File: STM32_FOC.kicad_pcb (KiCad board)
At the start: 2 copper layers, 26.5 x 26.5 mm, 46 parts, among them J1 Conn_01x07, J2 Conn_01x02, J3 Conn_01x03, J4 Conn_01x04, U1 STM32F103C8T6, U2 MP2359, U3 AS5600, U4 DRV8313, Y1 Crystal_GND3_Small

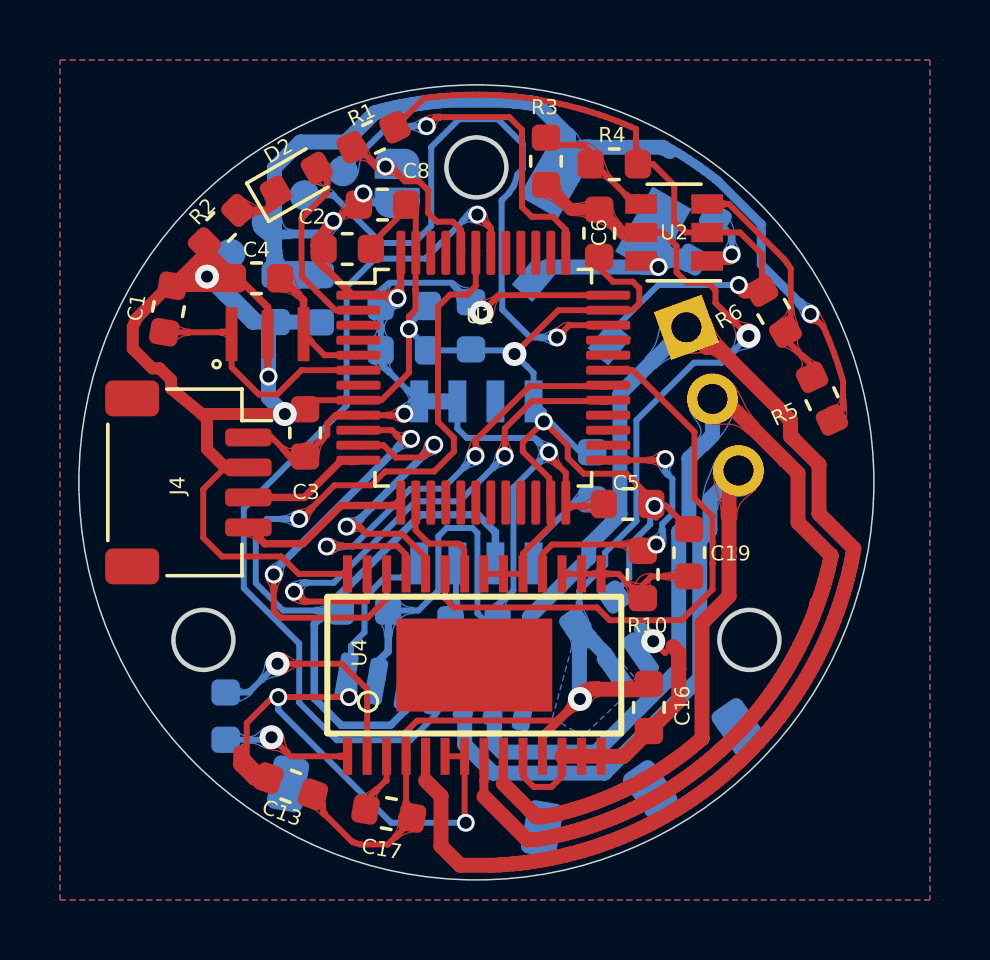
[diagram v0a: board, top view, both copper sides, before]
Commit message: first commit
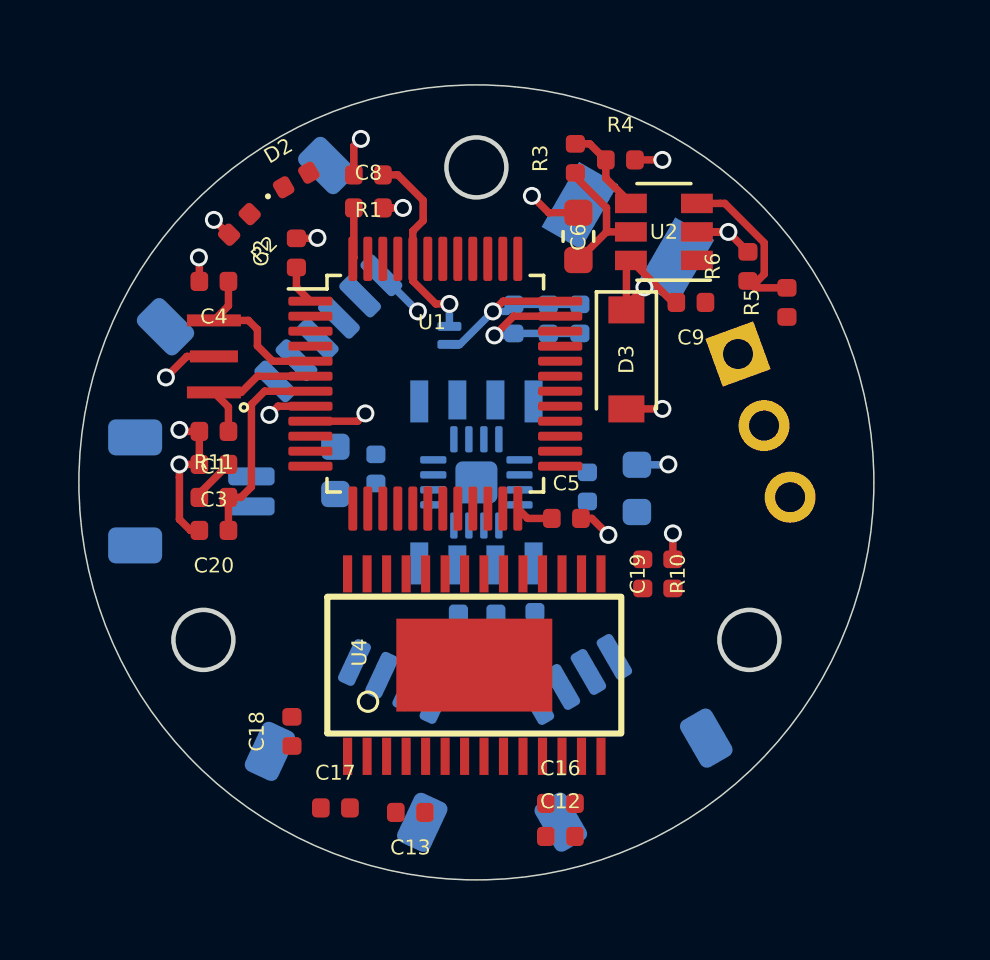
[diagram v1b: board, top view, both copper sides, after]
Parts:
- removed 3.3V, CLK, DIO, GND: TestPoint, TestPoint:TestPoint_Pad_D1.0mm
- added C20: 100nf, Capacitor_SMD:C_0402_1005Metric, F.Cu at (91.2, 101.6)
- added C21: 100nf, Capacitor_SMD:C_0402_1005Metric, B.Cu at (103.7, 100.2)
- added C22: 10uf, Capacitor_SMD:C_0603_1608Metric, B.Cu at (105.3, 100.2)
- added J5: Conn_01x06, Connector_JST:JST_SH_SM06B-SRSS-TB_1x06-1MP_P1.00mm_Horizontal, B.Cu at (93.7, 93.5)
- added R11: 10K, Resistor_SMD:R_0402_1005Metric, F.Cu at (91.2, 100.5)
- C1, C10, C11, C13, C16, C17, C2, C3, C4, C5, C7, C8: footprint Capacitor_SMD:C_0603_1608Metric -> Capacitor_SMD:C_0402_1005Metric
- C12, C18, C9: footprint Capacitor_SMD:C_0603_1608Metric -> Capacitor_SMD:C_0402_1005Metric; moved to F.Cu
- C14: value 0.1uf -> 100nf; footprint Capacitor_SMD:C_0603_1608Metric -> Capacitor_SMD:C_0402_1005Metric
- C19: value 100uf -> 0.47uf; footprint Capacitor_SMD:C_0603_1608Metric -> Capacitor_SMD:C_0402_1005Metric
- D2: footprint LED_SMD:LED_0603_1608Metric -> LED_SMD:LED_0402_1005Metric
- D3: moved to F.Cu
- J1: value Conn_01x07 -> Conn_01x04; footprint Connector_JST:JST_SH_SM07B-SRSS-TB_1x07-1MP_P1.00mm_Horizontal -> Connector_JST:JST_SH_SM04B-SRSS-TB_1x04-1MP_P1.00mm_Horizontal
- J4: moved to B.Cu
- JP1: footprint Jumper:SolderJumper-2_P1.3mm_Open_RoundedPad1.0x1.5mm -> Jumper:SoldJumper-2-P0.5mm_Open_RoundedPad
- R1, R10, R2, R3, R4, R5, R6, R7, R8, R9: footprint Resistor_SMD:R_0603_1608Metric -> Resistor_SMD:R_0402_1005Metric
- moved J2 17.3 mm to (90.5, 100.3), turned to 90 degrees
- moved J4 10.4 mm to (96.5, 108.5), turned to 155 degrees
- moved C11 10.2 mm to (103.5, 94.5)
- moved C10 7.65 mm to (102.4, 94.5)
- moved C12 7.62 mm to (102.8, 111.8), turned to 0 degrees
- moved J1 6.05 mm to (104.3, 108.3), turned to 210 degrees
- moved C15 5.94 mm to (95.3, 99.6), turned to 90 degrees
- moved R8 5.37 mm to (102.0, 104.8)
- moved JP1 5.34 mm to (99.0, 95.1)
- moved C1 4.35 mm to (91.2, 98.3), turned to 180 degrees
- moved C16 4.35 mm to (102.8, 110.7), turned to 0 degrees
- moved C13 4.08 mm to (97.8, 111.0), turned to 180 degrees
- moved C14 4.06 mm to (96.7, 99.5), turned to 90 degrees
- moved R5 3.42 mm to (110.3, 94.0), turned to 90 degrees
- moved C3 3.22 mm to (91.2, 99.4), turned to 180 degrees
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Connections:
- net Net-(U1-Pad32) renamed USB_DM
- net Net-(U1-Pad33) renamed USB_DP
- D3 pad 1: GND -> Net-(C9-Pad2)
- D3 pad 2: Net-(C9-Pad2) -> GND
- J1 pad 1: U -> SWDIO
- J1 pad 2: V -> SWCLK
- J1 pad 3: W -> +3V3
- J1 pad 4: I2C1_SCL -> GND
- R8 pad 1: Net-(R8-Pad1) -> GND
- R8 pad 2: GND -> Net-(R8-Pad2)
- U1 pad 11: EN2 -> Net-(U1-Pad11)
- U1 pad 14: EN3 -> CS
- U1 pad 15: Net-(U1-Pad15) -> SCK
- U1 pad 16: Net-(U1-Pad16) -> MISO
- U1 pad 17: Net-(U1-Pad17) -> MOSI
- U1 pad 18: Net-(U1-Pad18) -> A
- U1 pad 19: Net-(U1-Pad19) -> B
- U1 pad 20: Net-(U1-Pad20) -> Z
- U1 pad 22: Net-(U1-Pad22) -> ERROR
- U1 pad 25: ERROR -> SPI2_CS
- U1 pad 26: Net-(U1-Pad26) -> SPI2_SCK
- U1 pad 27: Net-(U1-Pad27) -> SPI2_MISO
- U1 pad 28: Net-(U1-Pad28) -> SPI2_MOSI
- U1 pad 7: NRST -> Net-(C20-Pad1)
- U3 pad 5: Net-(R8-Pad1) -> Net-(R8-Pad2)
- U4 pad 22: EN3 -> EN1
- U4 pad 24: EN2 -> EN1
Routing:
- net GND: track 169.4 -> 35.6 mm, vias 12 -> 18
- net +3V3: track 101.6 -> 15.8 mm, vias 7 -> 2
- net U: track 47.4 -> 0.14 mm
- net V: track 45.1 -> 0.00 mm
- net +12V: track 45.6 -> 4.53 mm, vias 2 -> 0
- net W: track 37.1 -> 0.00 mm
- net I2C1_SDA: track 36.1 -> 0.00 mm, vias 1 -> 0
- net I2C1_SCL: track 33.9 -> 0.00 mm, vias 1 -> 0
- net SWDIO: track 21.4 -> 0.00 mm, vias 1 -> 0
- net PWMC: track 19.7 -> 0.00 mm
- net PWMA: track 17.1 -> 0.00 mm, vias 2 -> 0
- net PWMB: track 15.3 -> 0.00 mm, vias 2 -> 0
- net EN1: track 14.5 -> 0.00 mm, vias 2 -> 0
- net SWCLK: track 12.0 -> 0.00 mm, vias 1 -> 0
- net EN2: track 10.5 -> 0.00 mm, vias 2 -> 0
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- added copper zone on In1.Cu, net GND
- removed copper zone on B.Cu, net +12V
- removed copper zone on B.Cu, net GND
- removed copper zone on F.Cu, net GND
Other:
- copper layers 2 -> 4
- net class Default: clearance 0.2 -> 0.1
- rule trace_clearance: 0.2 -> 0.1
